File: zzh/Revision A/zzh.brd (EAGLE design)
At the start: 34.4 x 13.8 mm, 37 parts, among them IC1 CC2652R1FRGZ, IC3 ME6211C33R5G, SW1 K2-1177SW-D4DW-06, U1 CH340E, Y1 32.768KHz, Y2 48.000MHz

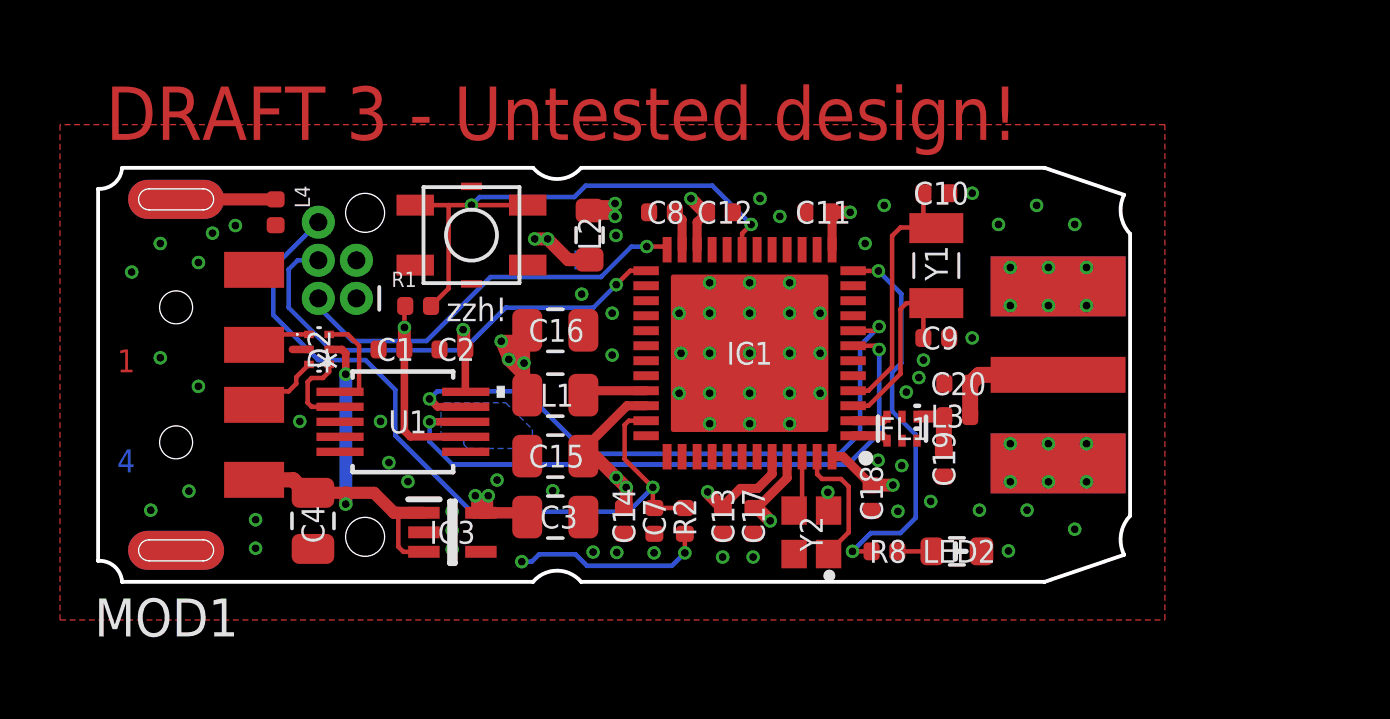
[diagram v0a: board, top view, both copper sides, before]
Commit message: zzh: Revision A release
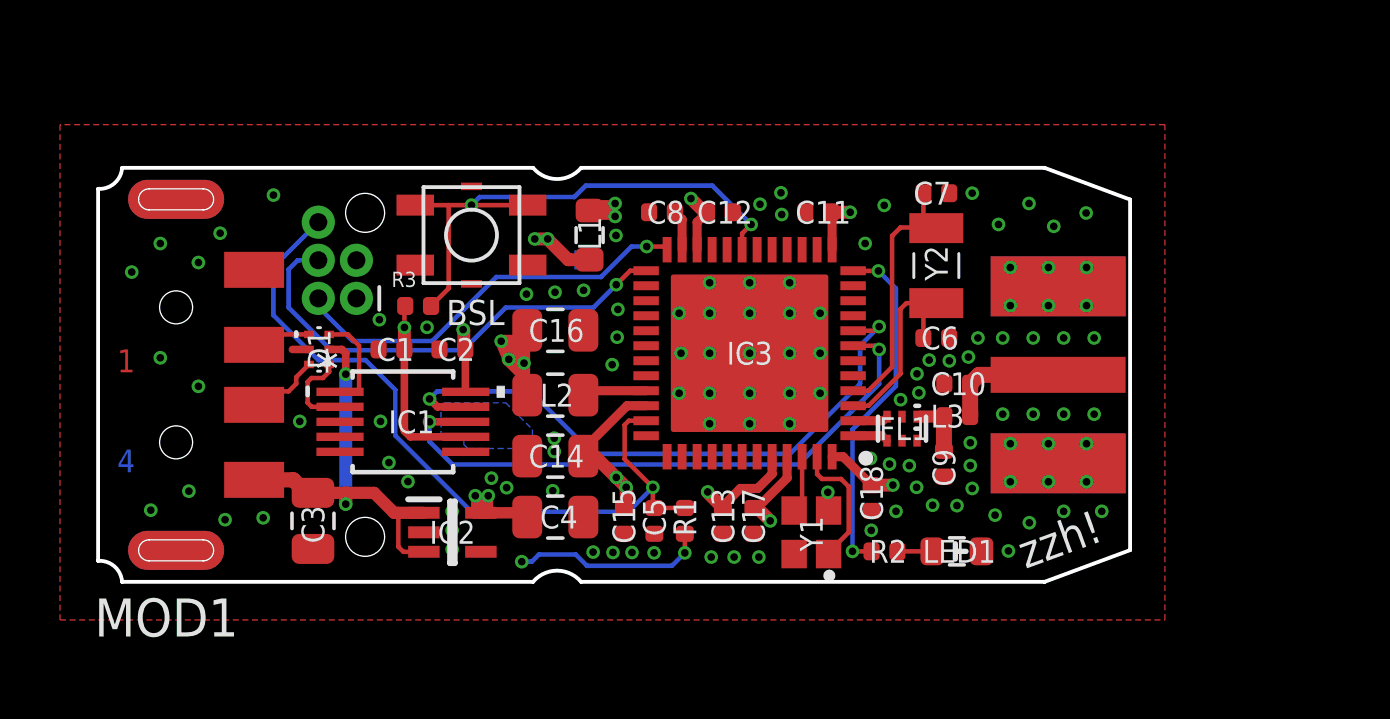
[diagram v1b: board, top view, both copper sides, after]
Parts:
- removed C19, C20: DNP, ok-discretes-dev:_PKG_C_0402
- removed L4: (no value), ok-discretes-dev:_PKG_L_0402
- removed R8: (no value), ok-discretes-dev:_PKG_C_0402
- removed U1: CH340E, ok-chips-dev:_PKG_MSOP10_TI-DGS10
- added C5: 100n, ok-discretes-dev:_PKG_C_0402
- added C6: 12p, ok-discretes-dev:_PKG_C_0402
- added IC2: ME6211C33R5G, ok-chips-dev:SOT65P212X110-5N
- added R3: 100K, ok-discretes-dev:_PKG_C_0402
- C10, C9: value 12p -> DNP
- C14: value 100n -> 22u; device ok-discretes-dev:_PKG_C_0402 -> ok-discretes-dev:_PKG_C_0805
- C15: value 22u -> 100n; device ok-discretes-dev:_PKG_C_0805 -> ok-discretes-dev:_PKG_C_0402
- C7: value 100n -> 12p
- CON3: value (none) -> DNP
- IC1: value CC2652R1FRGZ -> CH340E; device ok-chips-dev:QFN50P700X700X100-49N -> ok-chips-dev:_PKG_MSOP10_TI-DGS10
- IC3: value ME6211C33R5G -> CC2652R1FRGZ; device ok-chips-dev:SOT65P212X110-5N -> ok-chips-dev:QFN50P700X700X100-49N
- L1: value 6u8 -> BLM18HE152SN1; device ok-discretes-dev:_PKG_C_0805 -> ok-discretes-dev:_PKG_L_0603
- L2: value BLM18HE152SN1 -> MLZ2012N6R8LT000; device ok-discretes-dev:_PKG_L_0603 -> ok-discretes-dev:_PKG_C_0805
- L3: value (none) -> 0
- R1: value DNP -> 100K
- R2: value 100k -> 100
- Y1: value 32.768KHz -> Q22FA12800150; device ok-xtal-osc-dev:XTAL-2P-3215 -> ok-xtal-osc-dev:XTAL-4P-2016
- Y2: value 48.000MHz -> 32.768KHz; device ok-xtal-osc-dev:XTAL-4P-2016 -> ok-xtal-osc-dev:XTAL-2P-3215
- moved C7 14.4 mm to (27.9, 13.0), turned to 180 degrees
- moved IC1 11.8 mm to (10.2, 5.33), turned to 0 degrees
- moved IC3 11.6 mm to (21.7, 7.62), turned to 180 degrees
- moved R1 11.4 mm to (19.6, 2.03), turned to 270 degrees
- moved Y1 9.82 mm to (23.8, 1.65)
- moved Y2 9.82 mm to (27.9, 10.5)
- moved C3 8.08 mm to (7.16, 2.03), turned to 270 degrees
- moved C4 8.08 mm to (15.2, 2.16), turned to 0 degrees
- moved R2 6.73 mm to (26.2, 1.02), turned to 0 degrees
- moved C10 6.39 mm to (28.6, 6.60), turned to 0 degrees
- moved L1 5.46 mm to (16.4, 11.6), turned to 90 degrees
- moved L2 5.46 mm to (15.2, 6.22), turned to 180 degrees
- moved C9 4.20 mm to (28.2, 3.94), turned to 90 degrees
- moved C14 3.14 mm to (15.2, 4.19), turned to 180 degrees
- moved C15 3.14 mm to (17.5, 2.03), turned to 270 degrees
- renumbered CON1 to CON3, D2 to D1, LED2 to LED1
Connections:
- removed net N$1: L4.1, MOD1.USB_SHIELD_1, MOD1.USB_SHIELD_2
- net ANT: now also C10.2; no longer C20.2
- net BSL: now also IC3.19, R3.2; no longer IC1.19, R1.2
- net DCDC_SW: now also IC3.33, L2.1; no longer IC1.33, L1.1
- net DCOUPL: now also IC3.23; no longer IC1.23
- net GND: now also C5.1, C6.1, IC1.3, IC2.2, IC3.49, MOD1.USB_SHIELD_1, MOD1.USB_SHIELD_2, Y1.2, Y1.4; no longer C19.1, C20.1, IC1.49, IC3.2, L4.2, U1.3, Y2.2, Y2.4
- net LED: now also IC3.12, R2.1; no longer IC1.12, R8.1
- net N$16: now also R2.2; no longer R8.2
- net PC_RX: now also IC1.9, IC3.8; no longer IC1.8, U1.9
- net PC_TX: now also IC1.8, IC3.7; no longer IC1.7, U1.8
- net RESET: now also C5.2, IC3.35, R1.1; no longer C7.2, IC1.35, R2.1
- net RF_N: now also IC3.2; no longer IC1.2
- net RF_P: now also IC3.1; no longer IC1.1
- net TCK: now also IC3.25; no longer IC1.25
- net TMS: now also IC3.24; no longer IC1.24
- net UD+: now also IC1.1; no longer U1.1
- net UD-: now also IC1.2; no longer U1.2
- net UNBAL: now also C9.2; no longer C19.2
- net VCC: now also C4.1, IC1.10, IC1.7, IC2.5, L1.1, R1.2, R3.1; no longer C3.1, IC3.5, L2.1, R1.1, R2.2, U1.10, U1.7
- net VDDR: now also IC3.45, IC3.48, L2.2; no longer IC1.45, IC1.48, L1.2
- net VDDS: now also IC3.13, IC3.22, IC3.34, IC3.44, L1.2; no longer IC1.13, IC1.22, IC1.34, IC1.44, L2.2
- net VUSB: now also C3.1, IC2.1, IC2.3; no longer C4.1, IC3.1, IC3.3
- net X32K_Q1: now also C6.2, IC3.3, Y2.1; no longer C9.2, IC1.3, Y1.1
- net X32K_Q2: now also C7.2, IC3.4, Y2.2; no longer C10.2, IC1.4, Y1.2
- net X48M_N: now also IC3.46, Y1.3; no longer IC1.46, Y2.3
- net X48M_P: now also IC3.47, Y1.1; no longer IC1.47, Y2.1
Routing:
- net N$1: track 3.32 -> 0.00 mm
- net LED: track 13.1 -> 11.7 mm
- net PC_RX: track 21.7 -> 20.7 mm
- net PC_TX: track 21.3 -> 20.3 mm
- net GND: vias 83 -> 114
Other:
- outline, holes or cut-outs redrawn
- board text added: "BSL"
- board text added: "For evaluation only Not FCC approved for resale"
- board text removed: "DRAFT 3 - Untested design!"
